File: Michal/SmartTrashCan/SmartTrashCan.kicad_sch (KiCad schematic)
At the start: 36 parts, among them J1 USB_C_Receptacle_USB2.0_16P, J2 USB_C_Receptacle_USB2.0_16P, SW1 SW_Push, SW2 SW_Push, U1 ESP32-C6-WROOM-1, U2 AZ1117-3.3, U3 CP2102N-Axx-xQFN20

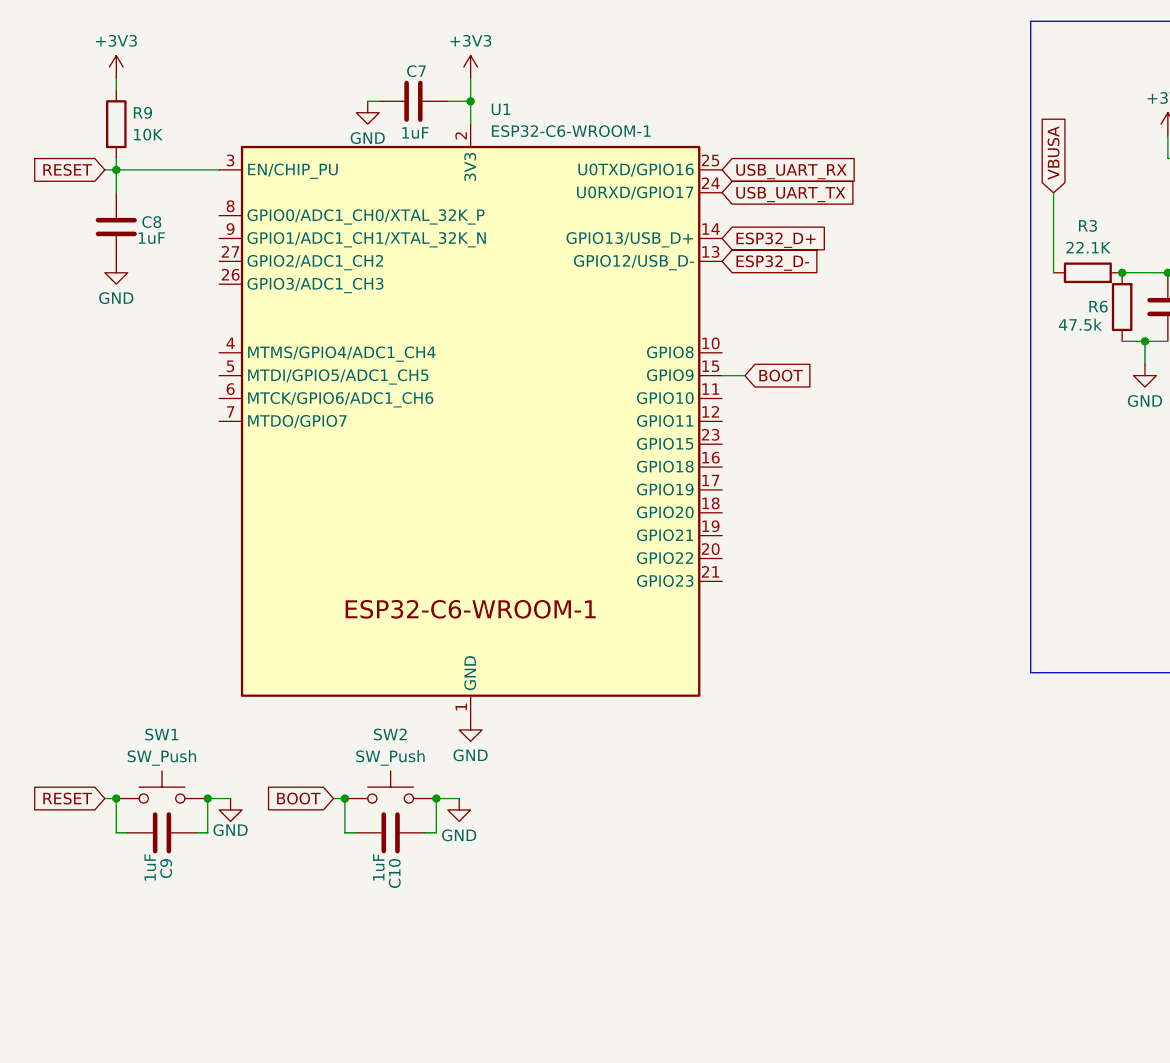
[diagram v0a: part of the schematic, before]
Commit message: Update SmartTrashCan.kicad_sch
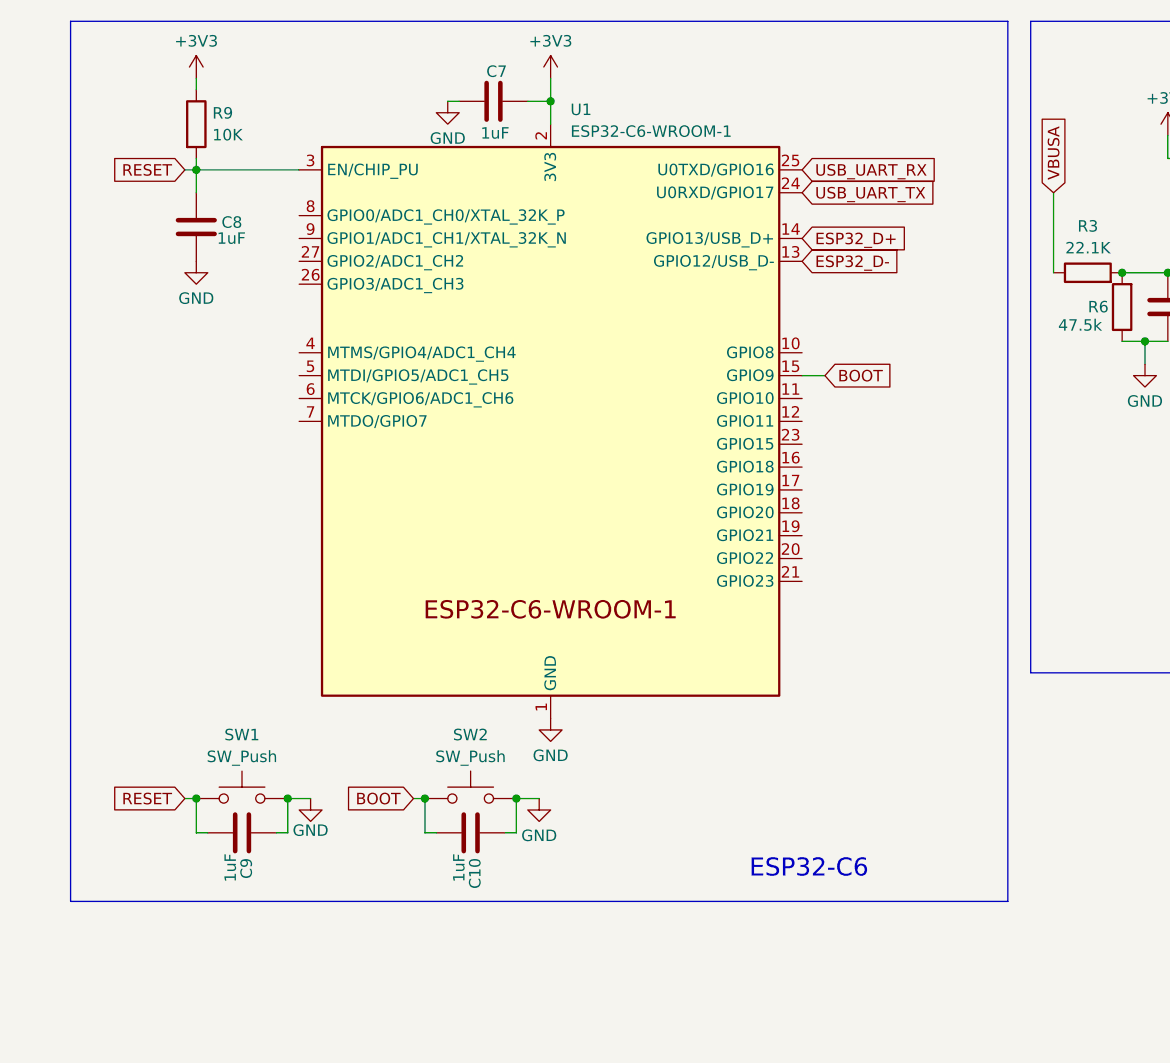
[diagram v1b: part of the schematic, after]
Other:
- note added: "ESP32-C6"
- moved on the sheet: C10, C7, C8, C9, R9, SW1, SW2, U1
